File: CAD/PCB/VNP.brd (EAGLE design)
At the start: 24.8 x 106.7 mm, 10 parts, among them U1 VR

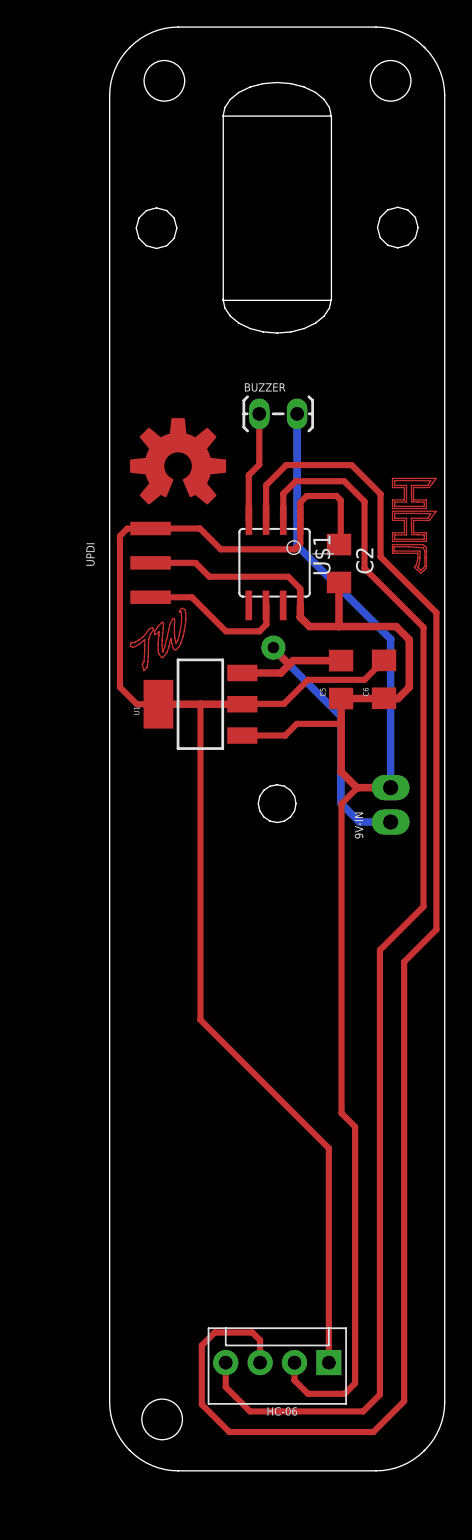
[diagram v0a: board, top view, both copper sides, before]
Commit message: Board Fix
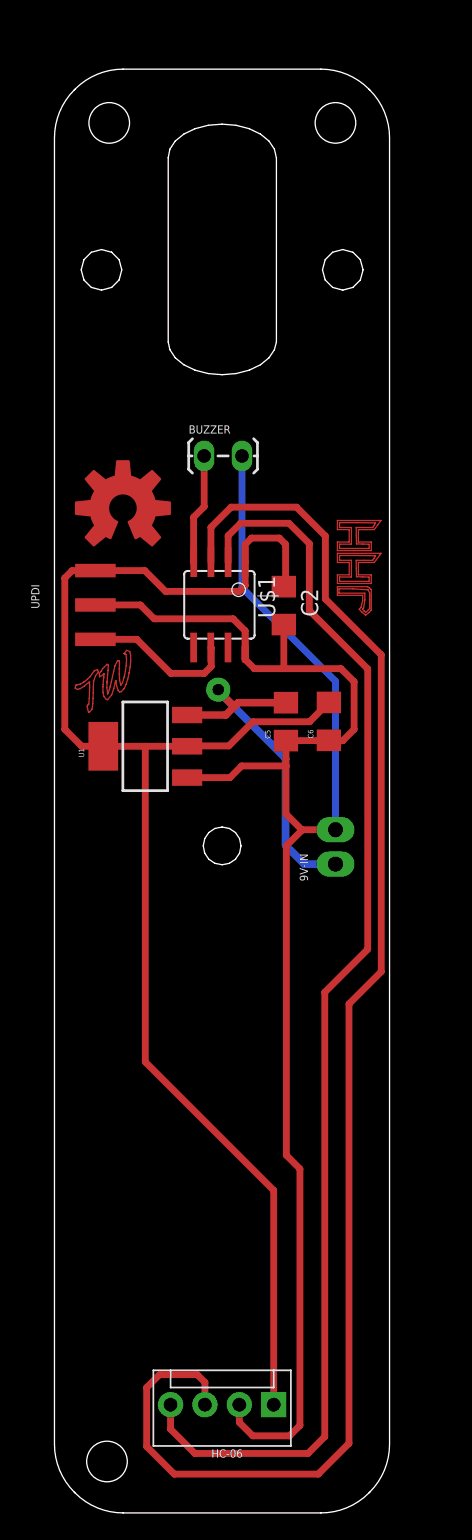
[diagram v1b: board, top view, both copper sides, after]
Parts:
- moved C6 5.13 mm to (20.4, 58.6)
- moved HC-06 5.13 mm to (16.3, 8.14)
- moved BUZZER 5.13 mm to (11.3, 78.2)
- moved C2 5.13 mm to (17.1, 67.2)
- moved UPDI 5.13 mm to (-1.85, 67.2)
- moved 9V-IN 5.13 mm to (20.9, 48.1)
- moved C5 5.13 mm to (17.2, 58.6)
- moved U1 5.13 mm to (6.83, 56.8)
- moved U$1 5.13 mm to (12.3, 67.2)
- moved U$2 5.13 mm to (5.18, 74.4)
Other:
- outline, holes or cut-outs redrawn
